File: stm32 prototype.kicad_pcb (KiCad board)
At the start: 4 copper layers, 149.5 x 46 mm, 120 parts, among them J1 USB_B_Mini, J10 Conn_01x15, J11 Conn_01x15, J2 Conn_01x06, J3 Conn_02x08_Odd_Even, J4 Conn_01x10, J5 Conn_02x04_Odd_Even, J6 Conn_01x15, J7 Conn_01x15, J8 Conn_01x15, J9 Conn_01x15, Q1 Q_NMOS_GSD, Q10 Q_NPN_BEC, Q11 Q_NMOS_GSD, Q2 Q_NMOS_GSD, Q3 Q_NMOS_GSD, Q4 Q_NMOS_GSD, Q5 Q_NMOS_GSD, Q6 Q_NMOS_GSD, Q7 Q_NMOS_GSD, Q8 Q_NMOS_GSD, Q9 Q_NPN_BEC, SW1 SW_Push, SW2 SW_Push, U1 FT232RL, U2 W25Q128JV-DTR, U3 STM32F407VGTx, U4 LD1117S33TR, U5 ESP32-WROOM, U7 TPS62203DBVR, Y1 Crystal_GND24

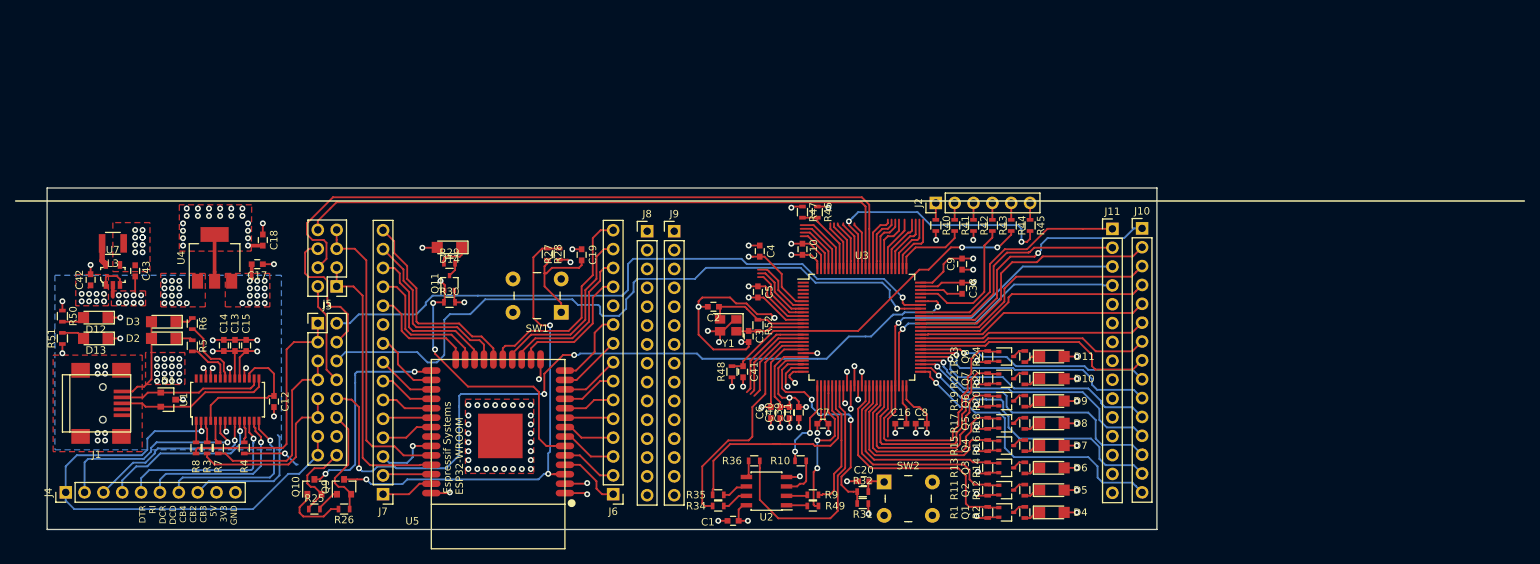
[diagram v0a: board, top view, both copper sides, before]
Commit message: Ordered PCB 12/18
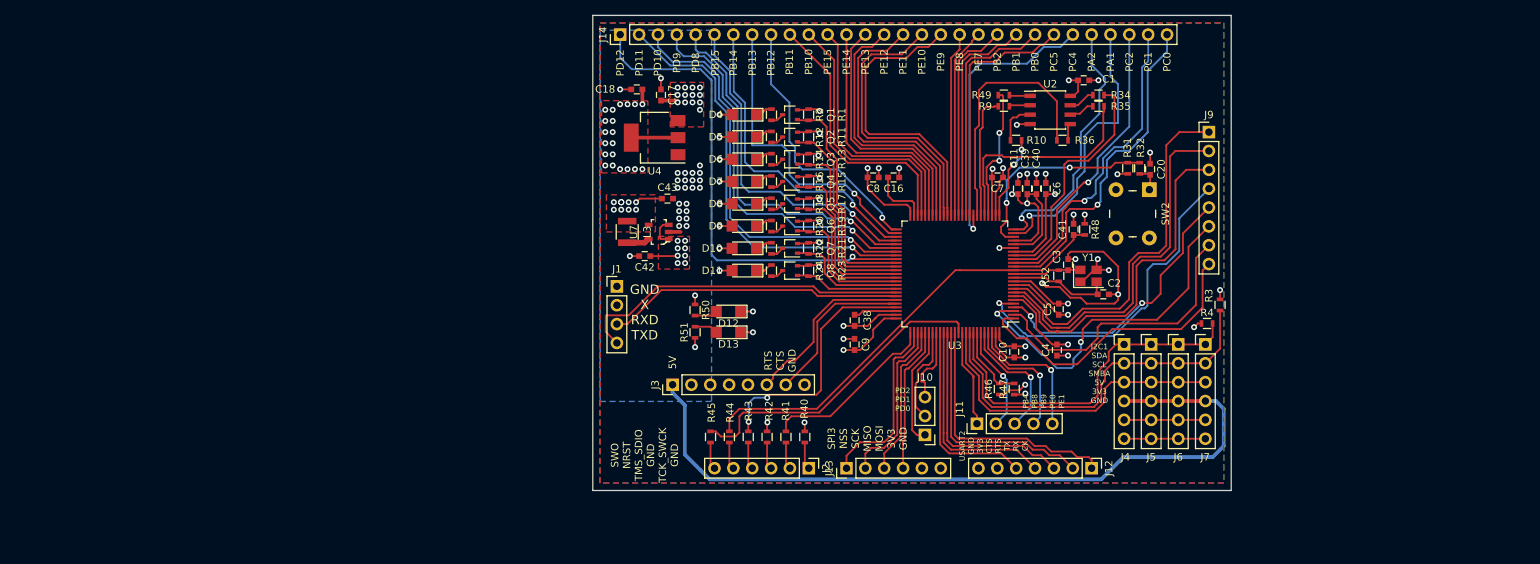
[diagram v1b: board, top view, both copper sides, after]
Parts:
- removed C12, C13, C14, C15: C, Capacitors_SMD:C_0603
- removed C19: 0.1uF, Capacitors_SMD:C_0603
- removed D1: SP0502BAHT, TO_SOT_Packages_SMD:SOT-23
- removed D14, D2, D3: LED, LEDs:LED_1206
- removed J8: Conn_01x15, Pin_Headers:Pin_Header_Straight_1x15_Pitch2.54mm
- removed Q10, Q9: Q_NPN_BEC, TO_SOT_Packages_SMD:SOT-23
- removed Q11: Q_NMOS_GSD, TO_SOT_Packages_SMD:SOT-323_SC-70
- removed R25, R26: 10k, Resistors_SMD:R_0603
- removed R27: 12k, Resistors_SMD:R_0603
- removed R28: 470R, Resistors_SMD:R_0603
- removed R29, R5, R6: 330R, Resistors_SMD:R_0603
- removed R30: 10K, Resistors_SMD:R_0603
- removed R7, R8: 0R, Resistors_SMD:R_0603
- removed SW1: SW_Push, switches_mdg:Switch_Tactile_6x6mm_Vertical_SMD_MJTP1230
- removed U1: FT232RL, Housings_SSOP:TSSOP-28_4.4x9.7mm_Pitch0.65mm
- removed U5: ESP32-WROOM, ESP32-footprints-Lib:ESP32-WROOM
- added J12: Conn_01x07, Pin_Headers:Pin_Header_Straight_1x07_Pitch2.54mm, F.Cu at (203.2, 127.0)
- added J13: Conn_01x06, Pin_Headers:Pin_Header_Straight_1x06_Pitch2.54mm, F.Cu at (170.2, 127.0)
- added J14: Conn_01x30, Pin_Headers:Pin_Header_Straight_1x30_Pitch2.54mm, F.Cu at (139.7, 68.6)
- J1: value USB_B_Mini -> Conn_01x04; footprint Connectors:USB_Mini-B -> Pin_Headers:Pin_Header_Straight_1x04_Pitch2.54mm
- J10: value Conn_01x15 -> Conn_01x03; footprint Pin_Headers:Pin_Header_Straight_1x15_Pitch2.54mm -> Pin_Headers:Pin_Header_Straight_1x03_Pitch2.54mm
- J11: value Conn_01x15 -> Conn_01x05; footprint Pin_Headers:Pin_Header_Straight_1x15_Pitch2.54mm -> Pin_Headers:Pin_Header_Straight_1x05_Pitch2.54mm
- J3: value Conn_02x08_Odd_Even -> Conn_01x08; footprint Pin_Headers:Pin_Header_Straight_2x08_Pitch2.54mm -> Pin_Headers:Pin_Header_Straight_1x08_Pitch2.54mm
- J4: value Conn_01x10 -> Conn_01x06; footprint Pin_Headers:Pin_Header_Straight_1x10_Pitch2.54mm -> Pin_Headers:Pin_Header_Straight_1x06_Pitch2.54mm
- J5: value Conn_02x04_Odd_Even -> Conn_01x06; footprint Pin_Headers:Pin_Header_Straight_2x04_Pitch2.54mm -> Pin_Headers:Pin_Header_Straight_1x06_Pitch2.54mm
- J6, J7: value Conn_01x15 -> Conn_01x06; footprint Pin_Headers:Pin_Header_Straight_1x15_Pitch2.54mm -> Pin_Headers:Pin_Header_Straight_1x06_Pitch2.54mm
- J9: value Conn_01x15 -> Conn_01x08; footprint Pin_Headers:Pin_Header_Straight_1x15_Pitch2.54mm -> Pin_Headers:Pin_Header_Straight_1x08_Pitch2.54mm
- R3, R4: value 0R -> 10K
- moved J4 144.0 mm to (207.6, 110.3), turned to 0 degrees
- moved R3 137.8 mm to (220.5, 105.0), turned to 270 degrees
- moved R4 130.8 mm to (218.8, 107.5), turned to 0 degrees
- moved J7 112.6 mm to (218.5, 110.3), turned to 0 degrees
- moved J5 110.0 mm to (211.2, 110.3), turned to 0 degrees
- moved D12 85.2 mm to (154.3, 105.9)
- moved D13 85.2 mm to (154.3, 108.7)
- moved R50 85.2 mm to (149.8, 105.7)
- moved R51 85.2 mm to (149.8, 108.7)
- moved J6 78.8 mm to (214.9, 110.3), turned to 0 degrees
- moved C1 75.8 mm to (202.1, 74.7), turned to 0 degrees
- moved R34 75.4 mm to (204.1, 76.7), turned to 180 degrees
- moved C42 74.7 mm to (143.0, 98.4), turned to 180 degrees
- moved U7 73.8 mm to (144.9, 95.2), turned to 90 degrees
- moved J9 73.3 mm to (219.0, 81.7)
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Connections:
- net ST_MISO renamed SPI1_MISO
- net ST_MOSI renamed SPI1_MOSI
- net ST_SCK renamed SPI1_SCK
- J1 pad 1: +5V -> GND
- J1 pad 2: Net-(D1-Pad1) -> (no net)
- J1 pad 3: Net-(D1-Pad2) -> FTDI_ST_TXD
- J1 pad 4: (no net) -> FTDI_ST_RXD
- J10 pad 1: PC8 -> PD0
- J10 pad 2: PC7 -> PD1
- J10 pad 3: PC6 -> PD2
- J11 pad 1: PA8 -> PB4
- J11 pad 2: PC9 -> PB8
- J11 pad 3: PB10 -> PB9
- J11 pad 4: PB11 -> PE0
- J11 pad 5: (no net) -> PE1
- J3 pad 1: Net-(J3-Pad1) -> +5V
- J3 pad 2: FTDI_ST_TXD -> (no net)
- J3 pad 3: Net-(J3-Pad1) -> (no net)
- J3 pad 4: FTDI_ES_TXD -> (no net)
- J3 pad 5: Net-(J3-Pad5) -> (no net)
- J3 pad 6: FTDI_ST_RXD -> FTDI_ST_RTS
- J3 pad 7: Net-(J3-Pad5) -> FTDI_CTS
- J3 pad 8: FTDI_ES_RXD -> GND
- J4 pad 1: Net-(J3-Pad13) -> I2C1_SDA
- J4 pad 2: FTDI_RI -> I2C1_SCL
- J4 pad 3: FTDI_DCR -> I2C1_SMBA
- J4 pad 4: FTDI_DCD -> +5V
- J4 pad 5: FTDI_CBUS4 -> +3V3
- J4 pad 6: FTDI_CBUS2 -> GND
- J5 pad 1: Net-(J5-Pad1) -> I2C1_SDA
- J5 pad 2: FTDI_ES_RXD -> I2C1_SCL
- J5 pad 3: Net-(J5-Pad1) -> I2C1_SMBA
- J5 pad 4: ST_ESP_RXD -> +5V
- J5 pad 5: Net-(J5-Pad5) -> +3V3
- J5 pad 6: FTDI_ES_TXD -> GND
- J6 pad 1: SENSOR_VP -> I2C1_SDA
- J6 pad 2: SENSOR_VN -> I2C1_SCL
- J6 pad 3: IO35 -> I2C1_SMBA
- J6 pad 4: IO32 -> +5V
- J6 pad 5: IO33 -> +3V3
- J6 pad 6: IO25 -> GND
- J7 pad 1: IO23 -> I2C1_SDA
- J7 pad 2: IO22 -> I2C1_SCL
- J7 pad 3: IO21 -> I2C1_SMBA
- J7 pad 4: IO19 -> +5V
- J7 pad 5: IO18 -> +3V3
- J7 pad 6: IO5 -> GND
- J9 pad 1: (no net) -> PC15
- J9 pad 2: (no net) -> PC14
- J9 pad 3: (no net) -> PC13
- J9 pad 4: (no net) -> PE6
- J9 pad 5: (no net) -> PE5
- J9 pad 6: (no net) -> PE4
- J9 pad 7: (no net) -> PE3
- J9 pad 8: (no net) -> PE2
- R3 pad 1: Net-(J3-Pad11) -> +3V3
- R3 pad 2: Net-(R3-Pad2) -> I2C1_SCL
- R4 pad 1: FTDI_CTS -> +3V3
- R4 pad 2: Net-(R4-Pad2) -> I2C1_SDA
- U3 pad 1: (no net) -> PE2
- U3 pad 15: (no net) -> PC0
- U3 pad 16: (no net) -> PC1
- U3 pad 17: (no net) -> PC2
- U3 pad 2: (no net) -> PE3
- U3 pad 24: (no net) -> PA1
- U3 pad 25: (no net) -> PA2
- U3 pad 3: (no net) -> PE4
- U3 pad 33: (no net) -> PC4
- U3 pad 34: (no net) -> PC5
- U3 pad 35: (no net) -> PB0
- U3 pad 36: (no net) -> PB1
- U3 pad 37: (no net) -> PB2
- U3 pad 38: (no net) -> PE7
- U3 pad 39: STATUS_BIT0 -> PE8
- U3 pad 4: (no net) -> PE5
- U3 pad 40: STATUS_BIT1 -> PE9
- U3 pad 41: STATUS_BIT2 -> PE10
- U3 pad 42: STATUS_BIT3 -> PE11
- U3 pad 43: STATUS_BIT4 -> PE12
- U3 pad 44: STATUS_BIT5 -> PE13
- U3 pad 45: STATUS_BIT6 -> PE14
- U3 pad 46: STATUS_BIT7 -> PE15
- U3 pad 5: (no net) -> PE6
- U3 pad 60: PD13 -> STATUS_BIT0
- U3 pad 61: PD14 -> STATUS_BIT1
- U3 pad 62: PD15 -> STATUS_BIT2
- U3 pad 63: PC6 -> STATUS_BIT3
- U3 pad 64: PC7 -> STATUS_BIT4
- U3 pad 65: PC8 -> STATUS_BIT5
- U3 pad 66: PC9 -> STATUS_BIT6
- U3 pad 67: PA8 -> STATUS_BIT7
- U3 pad 7: (no net) -> PC13
- U3 pad 77: (no net) -> SPI3_NSS
- U3 pad 78: (no net) -> SPI3_SCK
- U3 pad 79: (no net) -> SPI3_MISO
- U3 pad 8: (no net) -> PC14
- U3 pad 80: (no net) -> SPI3_MOSI
- U3 pad 81: (no net) -> PD0
- U3 pad 82: (no net) -> PD1
- U3 pad 83: (no net) -> PD2
- U3 pad 84: (no net) -> USART2_CTS
- U3 pad 85: (no net) -> USART2_RTS
- U3 pad 86: ST_ESP_RXD -> USART2_TX
- U3 pad 87: ST_ESP_TXD -> USART2_RX
- U3 pad 88: (no net) -> USART2_CK
- U3 pad 9: (no net) -> PC15
- U3 pad 90: (no net) -> PB4
- U3 pad 91: (no net) -> I2C1_SMBA
- U3 pad 92: (no net) -> I2C1_SCL
- U3 pad 93: (no net) -> I2C1_SDA
- U3 pad 95: (no net) -> PB8
- U3 pad 96: (no net) -> PB9
- U3 pad 97: (no net) -> PE0
- U3 pad 98: (no net) -> PE1
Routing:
- net (no net): track 220.7 -> 0.00 mm, vias 8 -> 0
- net ST_ESP_RXD: track 94.6 -> 0.00 mm
- net FTDI_ST_RTS: track 109.1 -> 24.2 mm, vias 4 -> 0
- net ST_ESP_TXD: track 84.6 -> 0.00 mm
- net Net-(J3-Pad13): track 67.2 -> 0.00 mm, vias 1 -> 0
- net ESP_EN: track 66.9 -> 0.00 mm, vias 3 -> 0
- net +5V: track 51.7 -> 116.1 mm, vias 42 -> 22
- net I2C1_SCL: track 0.00 -> 52.5 mm
- net PC15: track 0.00 -> 50.6 mm
- net PC14: track 0.00 -> 49.4 mm
- net FTDI_ST_RXD: track 94.7 -> 45.5 mm, vias 1 -> 0
- net I2C1_SDA: track 0.00 -> 48.7 mm
- net FTDI_ST_TXD: track 87.5 -> 39.9 mm, vias 1 -> 0
- net PE4: track 0.00 -> 47.3 mm, vias 0 -> 2
- net PC13: track 0.00 -> 46.8 mm
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- added copper zone on B.Cu, net GND
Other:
- board size 149.5 x 46 mm -> 86 x 64 mm
- rule pad_to_mask_clearance: 0.051 -> 0
- board text added: "5V"
- board text added: "GND X RXD TXD"
- board text added: "I2C1 SDA SCL SMBA 5V 3V3 GND"
- board text added: "PA1"
- board text added: "PA2"
- board text added: "PB0"
- board text added: "PB1"
- board text added: "PB10"
- board text added: "PB11"
- board text added: "PB12"
- board text added: "PB13"
- board text added: "PB14"
- board text added: "PB15"
- board text added: "PB2"
- board text added: "PB4 PB8 PB9 PE0 PE1"
- board text added: "PC0"
- board text added: "PC1"
- board text added: "PC2"
- board text added: "PC4"
- board text added: "PC5"
- board text added: "PD10"
- board text added: "PD11"
- board text added: "PD12"
- board text added: "PD2 PD1 PD0"
- board text added: "PD8"
- board text added: "PD9"
- board text added: "PE10"
- board text added: "PE11"
- board text added: "PE12"
- board text added: "PE13"
- board text added: "PE14"
- board text added: "PE15"
- board text added: "PE7"
- board text added: "PE8"
- board text added: "PE9"
- board text added: "RTS CTS GND"
- board text added: "SPI3 NSS SCK MISO MOSI 3V3 GND"
- board text added: "SWO NRST TMS_SDIO GND TCK_SWCK GND"
- board text added: "USART2 GND 3V3 CTS RTS TX RX CK"
- board text removed: "DTR RI DCR DCD CB4 CB2 CB3 5V 3V3 GND"
